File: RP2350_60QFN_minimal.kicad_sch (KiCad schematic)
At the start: 43 parts, among them J1 USB_B_Micro, J2 Conn_02x18_Odd_Even, J3 Conn_02x18_Odd_Even, J4 SM03B-SRSS-TB, SW1 SW_Push, SW2 SW_Push, U1 RP2350_60QFN, U2 NCP1117-3.3_SOT223, U3 W25Q128JVS, Y1 ABM8-272-T3

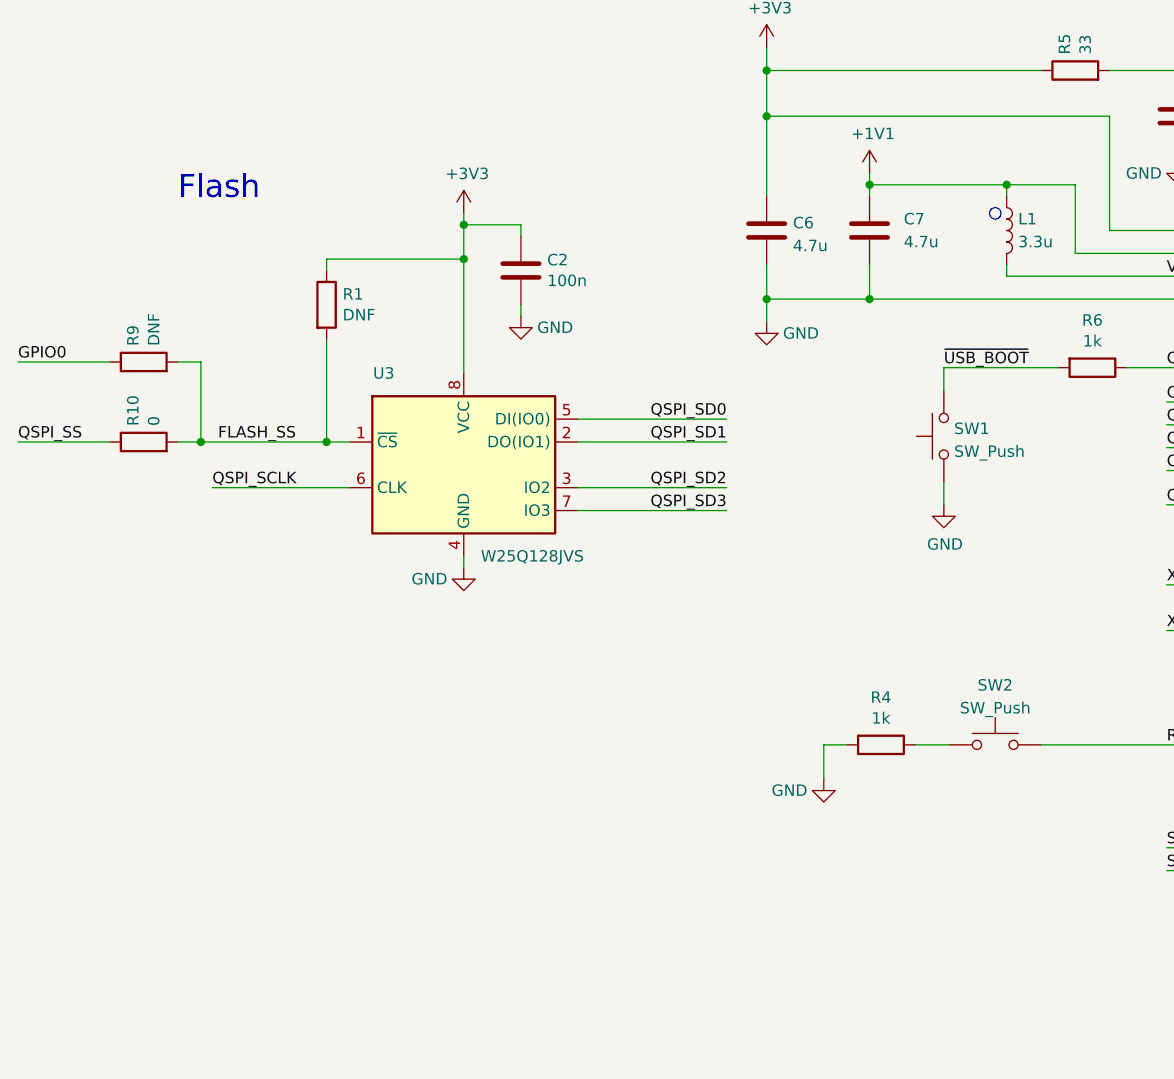
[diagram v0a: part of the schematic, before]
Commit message: update
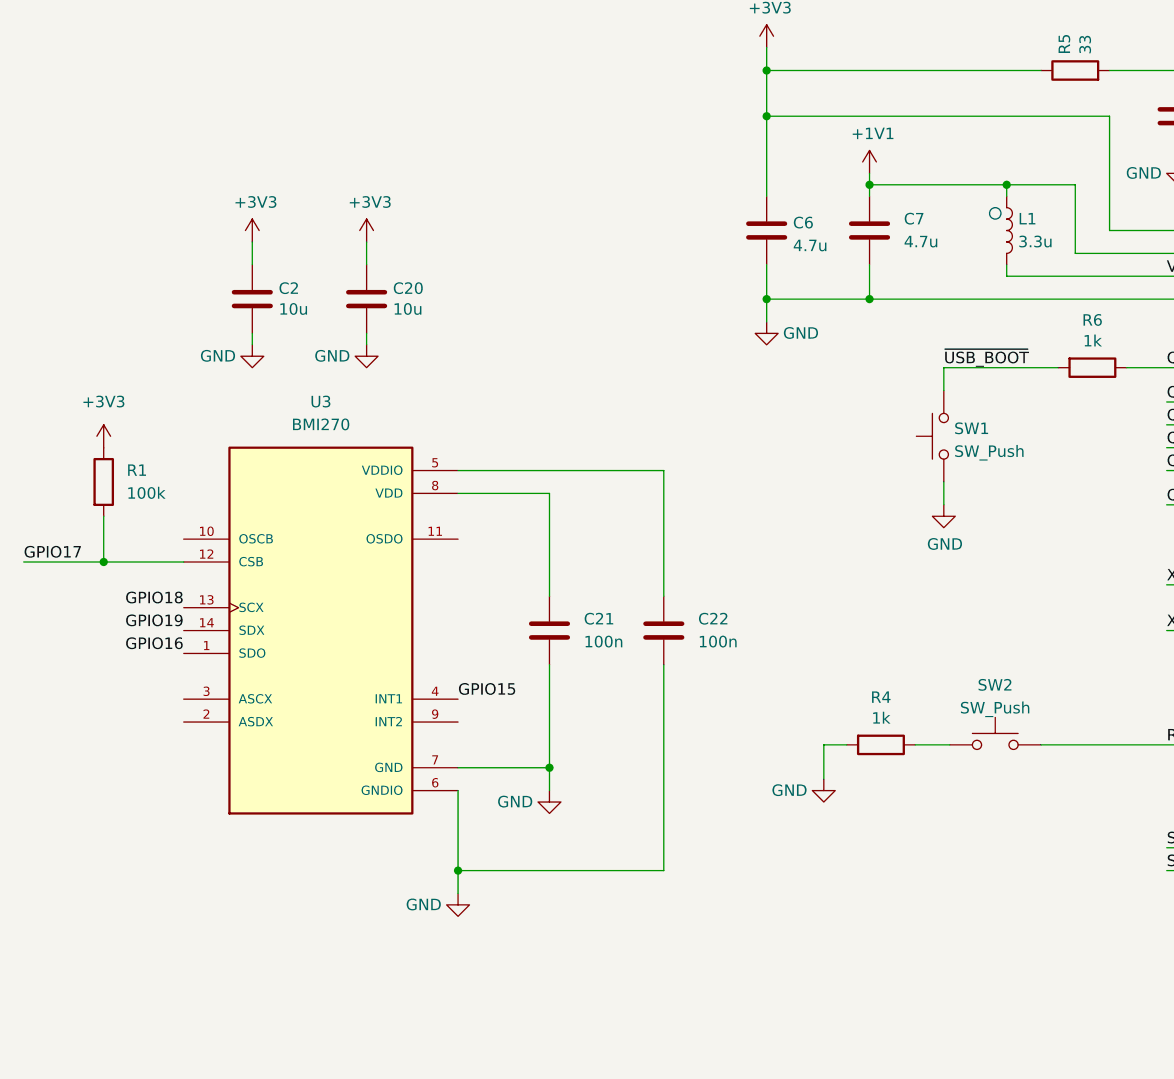
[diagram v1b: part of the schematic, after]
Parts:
- removed R10: 0, Resistor_SMD:R_0402_1005Metric, symbol Device:R
- removed R9: DNF, Resistor_SMD:R_0402_1005Metric, symbol Device:R
- removed U3: W25Q128JVS, Package_SO:SOIC-8_5.23x5.23mm_P1.27mm, symbol Memory_Flash:W25Q128JVS
- added C20: 10u, Capacitor_SMD:C_0805_2012Metric, symbol Device:C
- added C21, C22: 100n, symbol Device:C
- added U3: BMI270, BMI270:XDCR_BMI270, symbol BMI270:BMI270
- C2: value 100n -> 10u; footprint Capacitor_SMD:C_0402_1005Metric -> Capacitor_SMD:C_0805_2012Metric
- R1: value DNF -> 100k; footprint Resistor_SMD:R_0402_1005Metric -> (none)
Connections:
- net FLASH_SS is gone; now on net GPIO17: R1.2
- net +3V3: now also C20.1
- net GND: now also C20.2, C21.2, C22.2, U3.6 (GNDIO), U3.7 (GND)
- net GPIO15: now also U3.4 (INT1)
- net GPIO16: now also U3.1 (SDO)
- net GPIO17: now also U3.12 (CSB)
- net GPIO18: now also U3.13 (SCX)
- net GPIO19: now also U3.14 (SDX)
- new net: C22.1, U3.5 (VDDIO)
- new net: C21.1, U3.8 (VDD)
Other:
- note removed: "Flash"
